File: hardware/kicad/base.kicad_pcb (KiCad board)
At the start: 2 copper layers, 99.9 x 88.9 mm, 53 parts

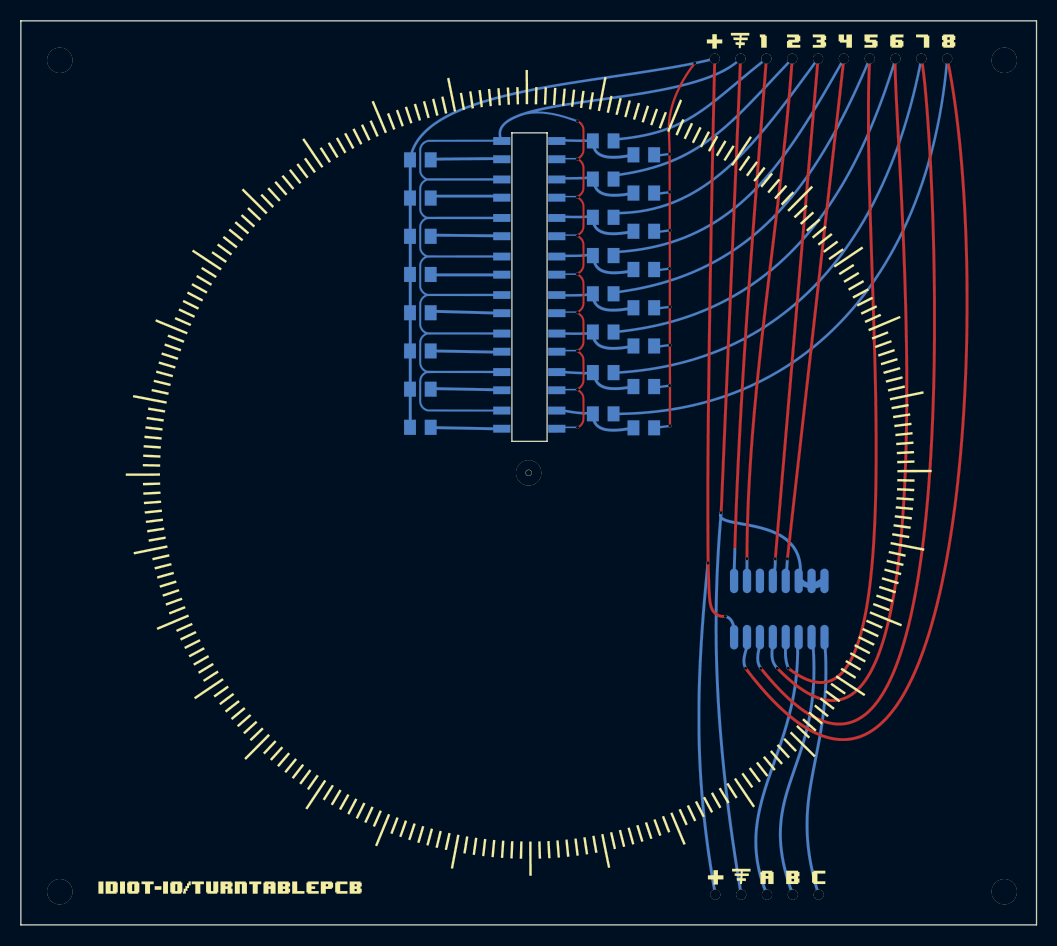
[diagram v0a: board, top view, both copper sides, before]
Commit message: i2c mux
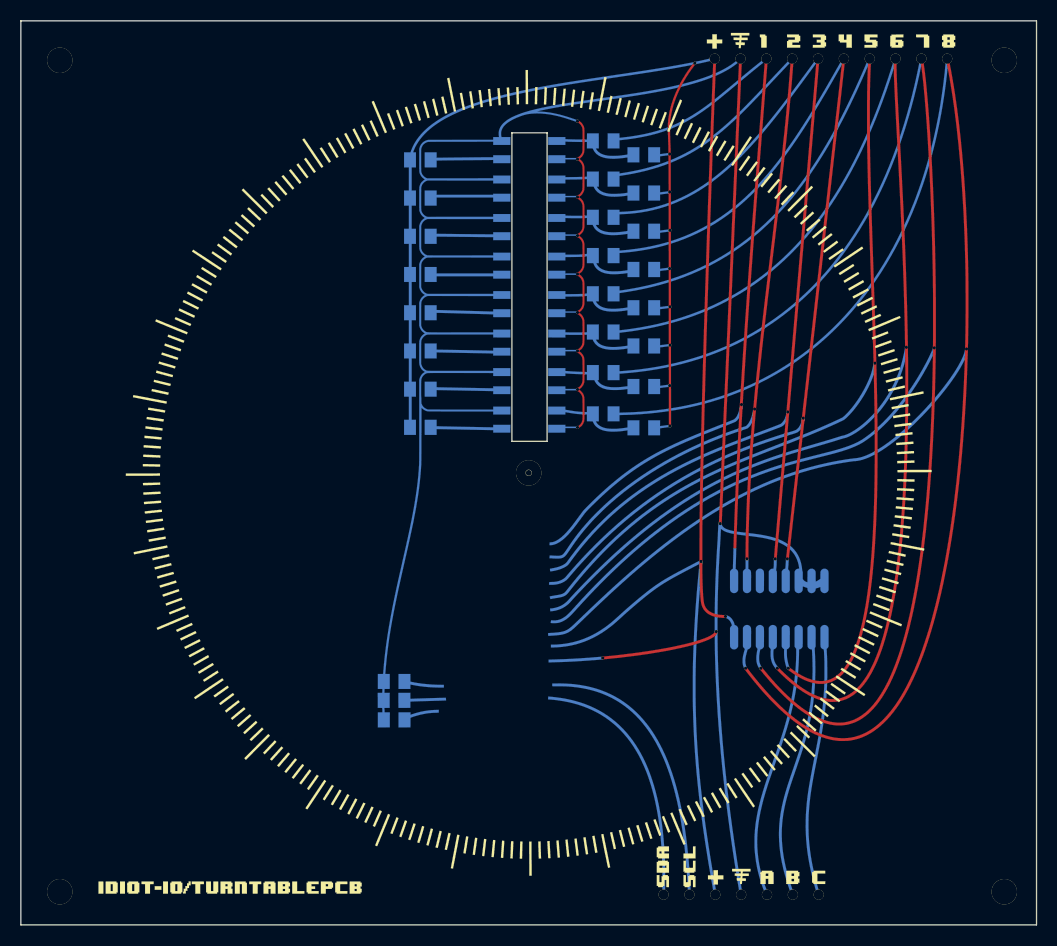
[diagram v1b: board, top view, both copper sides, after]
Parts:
- removed the ? at (19.0, 3.20)
- removed the ? at (17.7, 8.15)
- removed the G*** at (0.00, 0.00) (x5)
- added ?: , Wire_Pads:SolderWirePad_single_0-8mmDrill, F.Cu at (18.9, 4.27)
- added ?: , Wire_Pads:SolderWirePad_single_0-8mmDrill, F.Cu at (17.0, 8.00)
- added ?: , Wire_Pads:SolderWirePad_single_0-8mmDrill, F.Cu at (21.0, -7.43)
- added ?: , Wire_Pads:SolderWirePad_single_0-8mmDrill, F.Cu at (22.3, -6.99)
- added ?: , Wire_Pads:SolderWirePad_single_0-8mmDrill, F.Cu at (25.6, -6.70)
- added ?: , Wire_Pads:SolderWirePad_single_0-8mmDrill, F.Cu at (27.1, -6.10)
- added ?: , Wire_Pads:SolderWirePad_single_0-8mmDrill, F.Cu at (34.1, -11.5)
- added ?: , Wire_Pads:SolderWirePad_single_0-8mmDrill, F.Cu at (37.2, -13.1)
- added ?: , Wire_Pads:SolderWirePad_single_0-8mmDrill, F.Cu at (40.0, -13.0)
- added ?: , Wire_Pads:SolderWirePad_single_0-8mmDrill, F.Cu at (43.1, -12.9)
- added ?: , Wire_Pads:SolderWirePad_single_0-8mmDrill, F.Cu at (18.5, 14.9)
- added ?: , Wire_Pads:SolderWirePad_single_0-8mmDrill, F.Cu at (7.36, 17.5)
- added ?: , Wire_Pads:SolderWirePad_single_0-8mmDrill, F.Cu at (15.9, 40.8)
- added ?: , Wire_Pads:SolderWirePad_single_0-8mmDrill, F.Cu at (13.3, 40.8)
- added G*** (x5): LOGO, LOGO, F.Cu at (0.00, 0.00)
